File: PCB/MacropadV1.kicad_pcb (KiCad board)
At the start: 2 copper layers, 59 x 59 mm, 18 parts, among them J1 Conn_01x04, SW1 SW_Push, SW10 RotaryEncoder_Switch, SW2 SW_Push, SW3 SW_Push, SW4 SW_Push, SW5 SW_Push, SW6 SW_Push, U1 MOUDLE-SEEEDUINO-XIAO

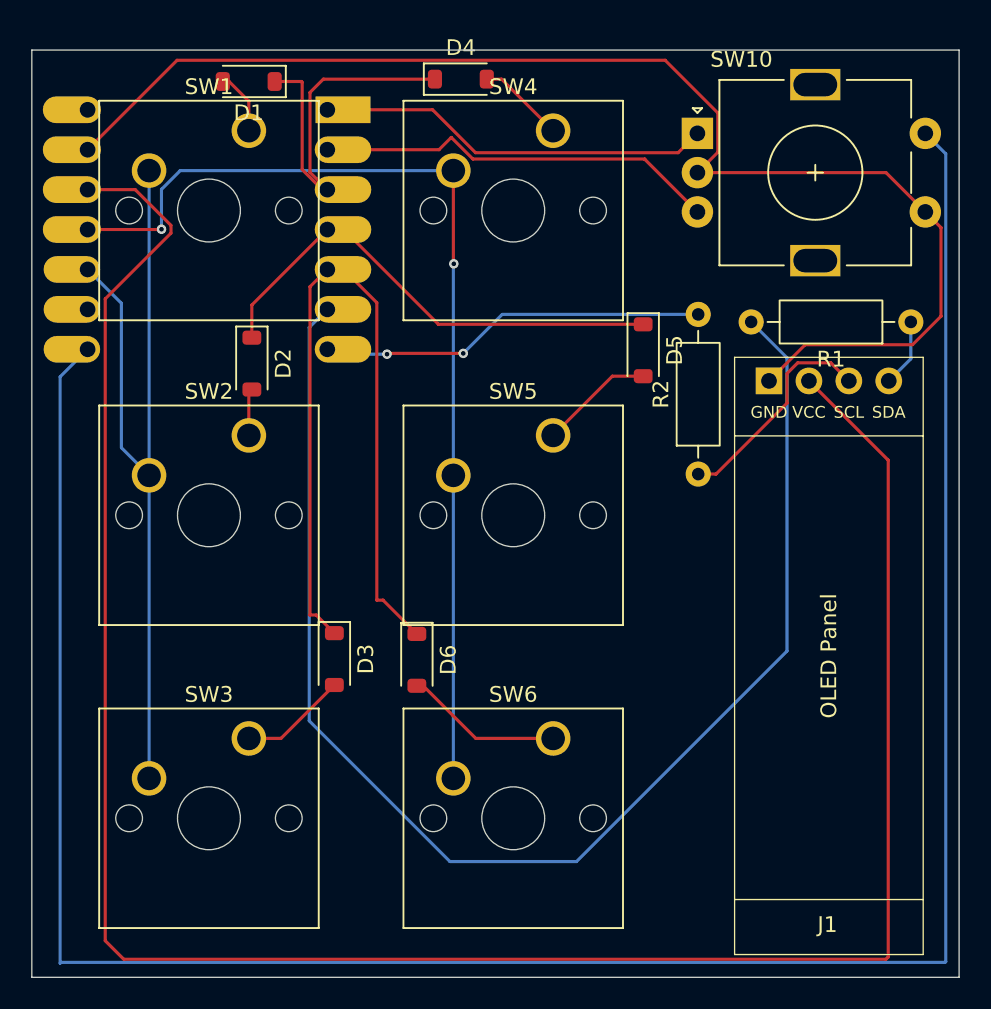
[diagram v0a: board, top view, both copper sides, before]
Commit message: added bom file
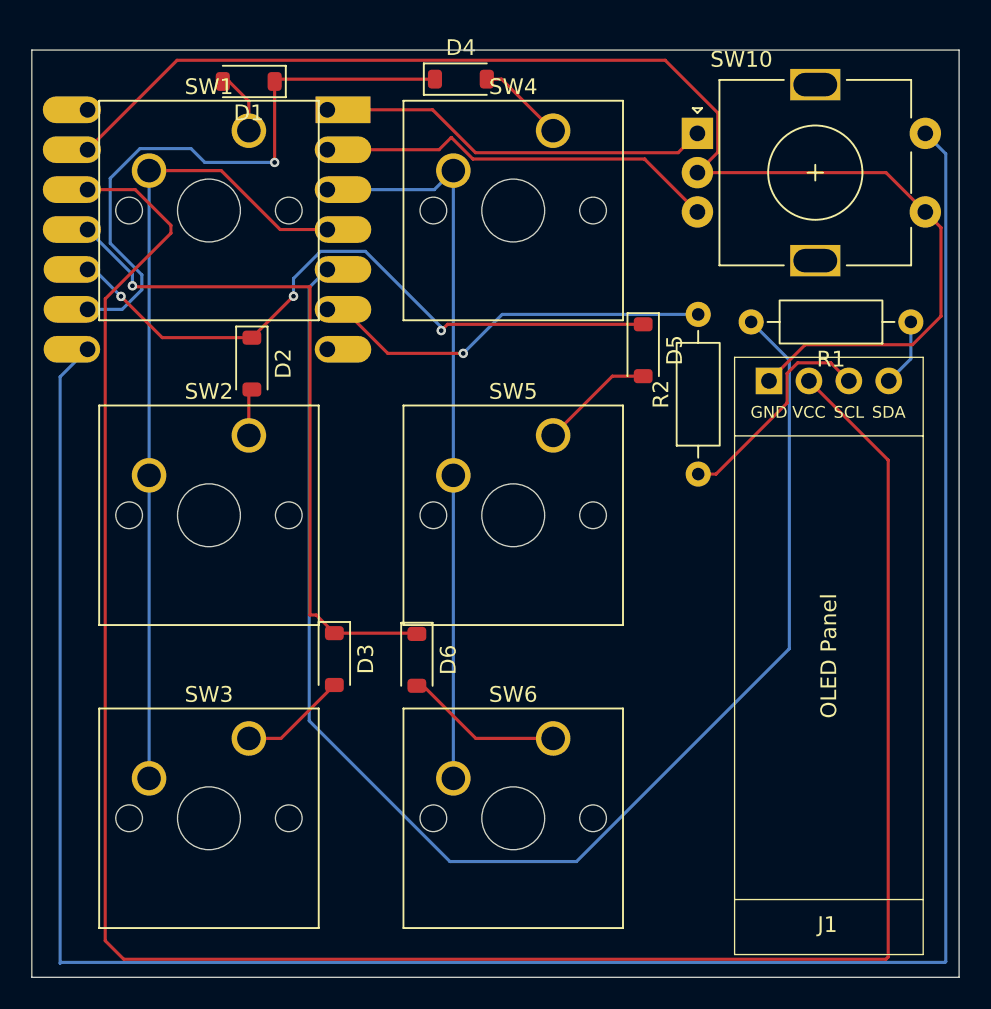
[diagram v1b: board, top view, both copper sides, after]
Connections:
- R1 pad 2: Net-(U1-PA9_A5_D5_SCL) -> Net-(U1-PA8_A4_D4_SDA)
- R2 pad 2: Net-(U1-PB08_A6_D6_TX) -> Net-(U1-PA9_A5_D5_SCL)
- U1 pad 10: col2 -> row2
- U1 pad 11: col1 -> row3
- U1 pad 3: row1 -> col1
- U1 pad 4: row2 -> col2
- U1 pad 5: row3 -> Net-(U1-PA8_A4_D4_SDA)
- U1 pad 7: Net-(U1-PB08_A6_D6_TX) -> unconnected-(U1-PB08_A6_D6_TX-Pad7)
- U1 pad 9: unconnected-(U1-PA7_A8_D8_SCK-Pad9) -> row1
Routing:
- net Net-(U1-PA8_A4_D4_SDA): track 0.00 -> 91.9 mm
- net Net-(U1-PA9_A5_D5_SCL): track 88.2 -> 25.8 mm, vias 0 -> 1
- net Net-(U1-PB08_A6_D6_TX): track 24.8 -> 0.00 mm, vias 2 -> 0
- net col1: track 65.0 -> 47.2 mm, vias 2 -> 0
- net row1: track 24.4 -> 38.9 mm, vias 0 -> 1
- net row2: track 31.5 -> 42.5 mm, vias 0 -> 3
- net row3: track 52.4 -> 44.3 mm, vias 0 -> 1
- net col2: track 53.4 -> 51.6 mm
